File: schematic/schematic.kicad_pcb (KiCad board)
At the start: 2 copper layers, 99.1 x 99.1 mm, 95 parts, among them J1 Peltier Connection, J2 USB_C_Receptacle_USB2.0, J3 Conn_01x01_Male, J4 Serial, J5 Conn_01x01_Male, J6 Conn_01x01_Male, J7 Conn_01x01_Male, J8 Conn_01x01_Male, SW1 Power Switch, U1 ESP32-D-WD-V3, U10 BSD316, U11 BSD316, U12 PC817, U13 PC817, U14 PC817, U15 AS431, U16 NL17SZ14, U17 XL6009, U18 slg55021, U19 XC9247B75CMR-G, U2 NL17SZ14, U20 MIC5211, U3 DMT3020LSDQ, U4 DMT3020LSDQ, U5 LM324, U6 slg55021, U7 NL17SZ14, U8 NL17SZ14, U9 BSD316, Y1 Crystal_GND24

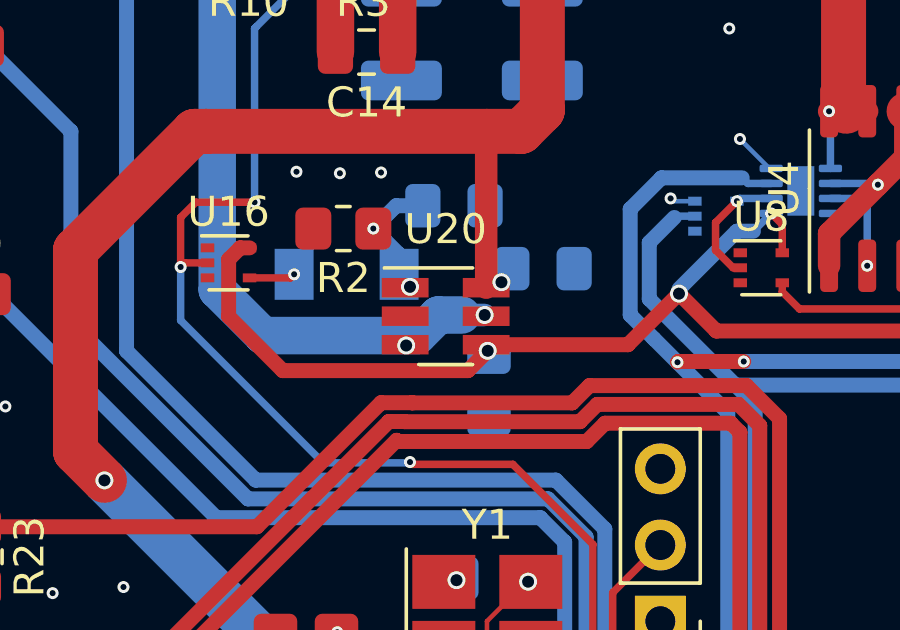
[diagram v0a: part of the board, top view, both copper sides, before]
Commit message: prelim ble working
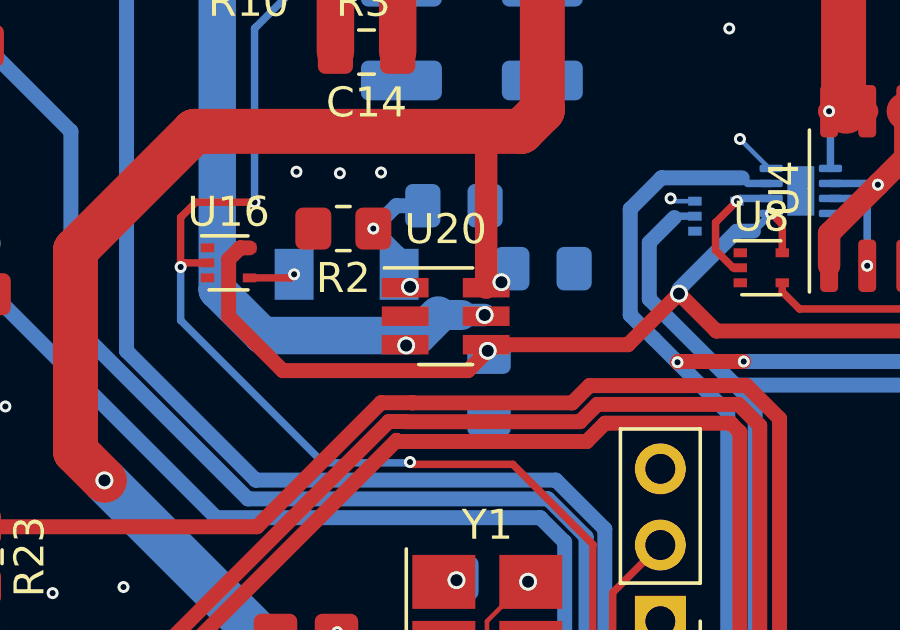
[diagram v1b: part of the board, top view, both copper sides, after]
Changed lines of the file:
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@@
   (segment (start 135.9662 53.3654) (end 136.9568 53.3654) (width 0.5) (layer "B.Cu") (net 77))
   (segment (start 114.5476 47.667) (end 124.0448 47.667) (width 1.5) (layer "B.Cu") (net 77))
-  (segment (start 138.3792 68.3514) (end 137.5918 68.3514) (width 1.25) (layer "B.Cu") (net 77))
+  (segment (start 138.3792 68.3514) (end 137.5918 68.3514) (width 1) (layer "B.Cu") (net 77))
   (segment (start 124.0448 47.667) (end 130.2258 53.848) (width 1.5) (layer "B.Cu") (net 77))
   (segment (start 130.2258 67.5132) (end 130.2258 53.848) (width 1.25) (layer "B.Cu") (net 77))
